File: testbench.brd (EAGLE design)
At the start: 100 x 100 mm, 47 parts, among them T1 C8492, T2 C8492, T3 C8545, T4 C8545, X1 MKDSN1,5/2-5,08

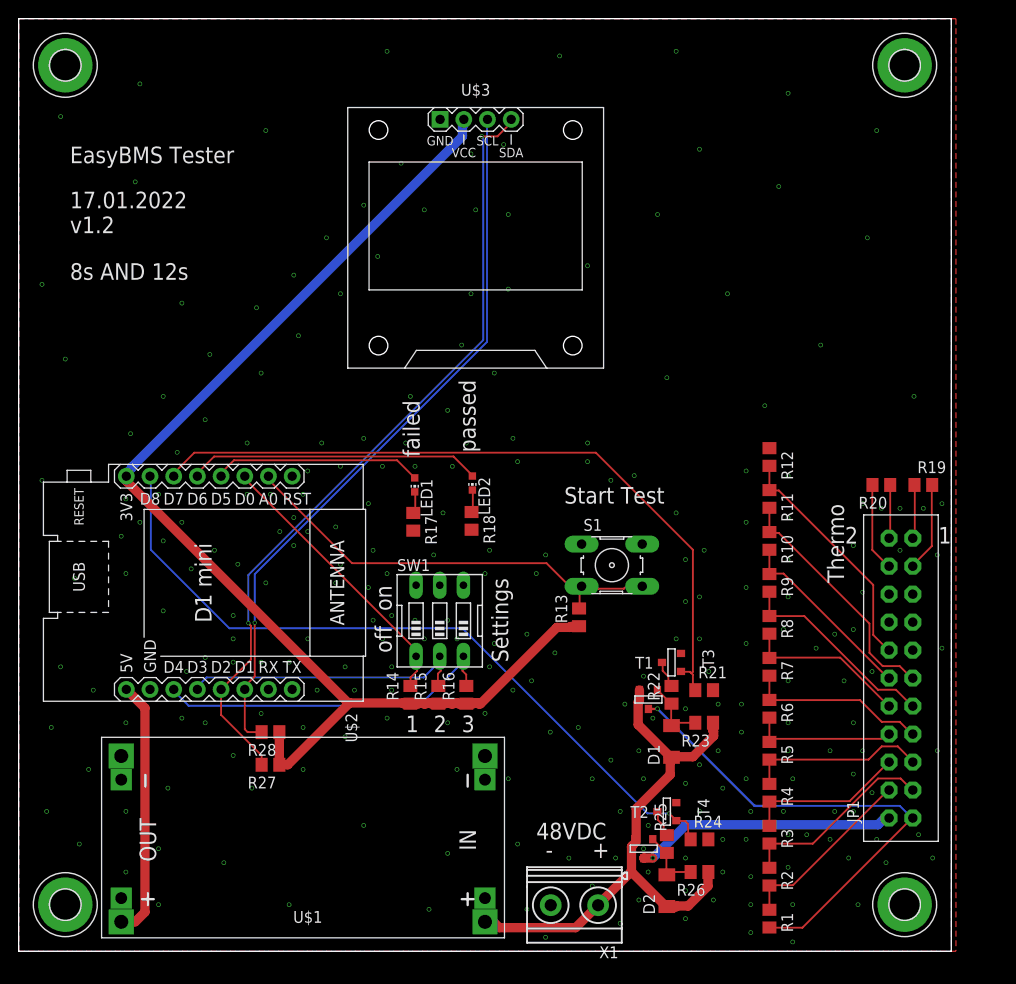
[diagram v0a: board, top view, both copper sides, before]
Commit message: new smd footprint of BMS connector integrated
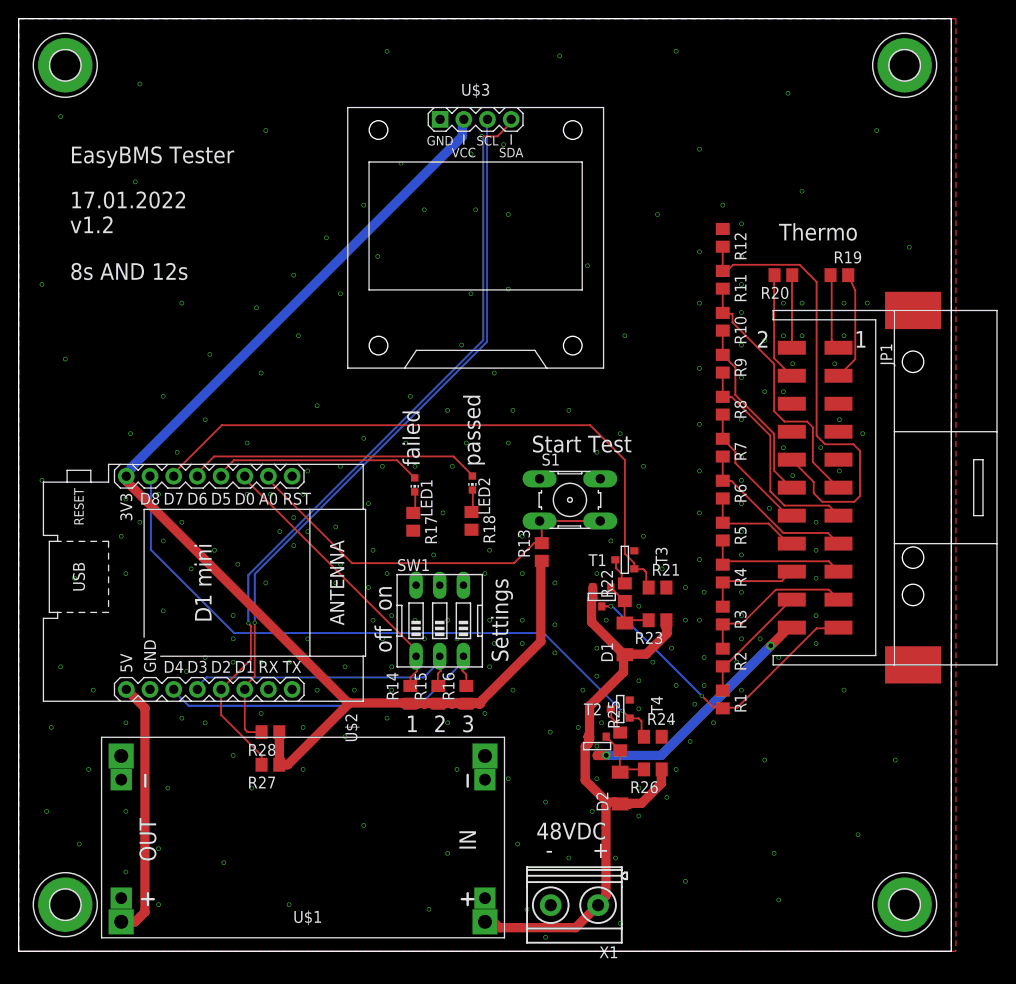
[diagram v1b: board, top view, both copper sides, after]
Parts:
- JP1: device pinhead_own:2X11_MEB12S_MODULSEITE -> pinhead_own:2X11_MEB12S_MODULSEITE_SMD
- moved R20 24.8 mm to (82.0, 72.5)
- moved R19 24.2 mm to (88.0, 72.5)
- moved R1 24.0 mm to (75.5, 27.0)
- moved R10 24.0 mm to (75.5, 67.5)
- moved R11 24.0 mm to (75.5, 72.0)
- moved R12 24.0 mm to (75.5, 76.5)
- moved R2 24.0 mm to (75.5, 31.5)
- moved R3 24.0 mm to (75.5, 36.0)
- moved R4 24.0 mm to (75.5, 40.5)
- moved R5 24.0 mm to (75.5, 45.0)
- moved R6 24.0 mm to (75.5, 49.5)
- moved R7 24.0 mm to (75.5, 54.0)
- moved R8 24.0 mm to (75.5, 58.5)
- moved R9 24.0 mm to (75.5, 63.0)
- moved JP1 21.5 mm to (87.9, 49.7), turned to 270 degrees
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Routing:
- net N$11: track 25.7 -> 50.5 mm
- net BATSIM: track 53.4 -> 33.5 mm, vias 1 -> 2
- net D7: track 77.7 -> 67.6 mm
- net D8: track 79.5 -> 70.0 mm
- net 48VDC: track 60.1 -> 67.5 mm
- net N$1: track 19.7 -> 13.0 mm
- net N$3: track 17.2 -> 10.5 mm
- net N$5: track 16.0 -> 11.3 mm
- net A0: track 48.0 -> 43.5 mm
- net N$2: track 21.4 -> 17.0 mm
- net +3V3: track 129.9 -> 133.9 mm
- net N$4: track 19.3 -> 15.7 mm
- net N$7: track 17.6 -> 14.1 mm
- net THERMO1IN: track 5.89 -> 8.14 mm
- net N$10: track 26.3 -> 28.5 mm
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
